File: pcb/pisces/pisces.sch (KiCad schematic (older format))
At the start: 41 parts, among them SW1 SW_PUSH, SW10 SW_PUSH, SW11 SW_PUSH, SW12 SW_PUSH, SW13 SW_PUSH, SW14 SW_PUSH, SW15 SW_PUSH, SW16 SW_PUSH, SW17 SW_PUSH, SW18 SW_PUSH, SW19 SW_PUSH, SW2 SW_PUSH, SW3 SW_PUSH, SW4 SW_PUSH, SW5 SW_PUSH, SW6 SW_PUSH, SW7 SW_PUSH, SW8 SW_PUSH, SW9 SW_PUSH, U1 ProMicro

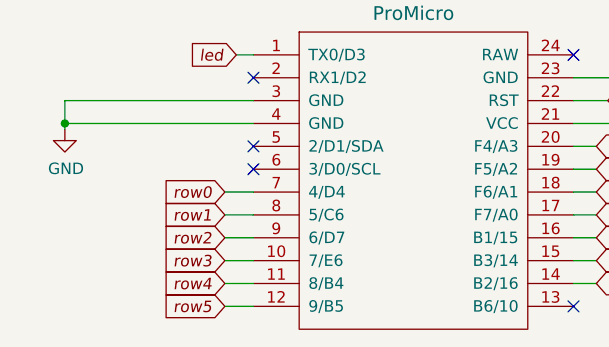
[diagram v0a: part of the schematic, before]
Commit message: Generated .net and .kicad_pcb
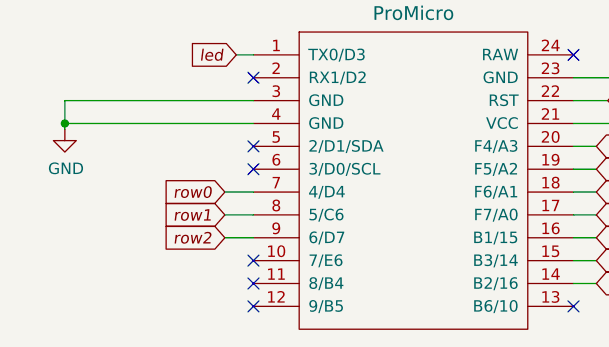
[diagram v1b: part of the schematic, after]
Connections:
- net row3: no longer names the net of U1.10 (7/E6)
- net row4: no longer names the net of U1.11 (8/B4)
- net row5: no longer names the net of U1.12 (9/B5)
- no-connect marks 6 -> 9
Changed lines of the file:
@@
 Pro Micro
-$Comp
-L kbd:ProMicro U1
-U 1 1 5FB09374
-P 2125 6925
-F 0 "U1" H 2125 7762 60  0000 C CNN
-F 1 "ProMicro" H 2125 7656 60  0000 C CNN
-F 2 "Keebio-Parts:ArduinoProMicro" H 2225 5875 60  0001 C CNN
-F 3 "" H 2225 5875 60  0000 C CNN
-	1    2125 6925
-	1    0    0    -1
-$EndComp
 $Comp
 L power:GND #PWR01
@@
 Text GLabel 1300 7175 0    50   Input Italic 0
 row2
-Text GLabel 1300 7275 0    50   Input Italic 0
-row3
-Text GLabel 1300 7375 0    50   Input Italic 0
-row4
-Text GLabel 1300 7475 0    50   Input Italic 0
-row5
 Text GLabel 2925 6775 2    50   Input Italic 0
 col0
@@
 Wire Wire Line
 	1300 7175 1425 7175
-Wire Wire Line
-	1300 7375 1425 7375
-Wire Wire Line
-	1300 7475 1425 7475
-Wire Wire Line
-	1300 7275 1425 7275
 NoConn ~ 2825 6375
 NoConn ~ 2825 7475
@@
 NoConn ~ 1425 6775
 NoConn ~ 1425 6475
+$Comp
+L kbd:ProMicro U1
+U 1 1 5FB09374
+P 2125 6925
+F 0 "U1" H 2125 7762 60  0000 C CNN
+F 1 "ProMicro" H 2125 7656 60  0000 C CNN
+F 2 "Keebio-Parts:ArduinoProMicro" H 2225 5875 60  0001 C CNN
+F 3 "" H 2225 5875 60  0000 C CNN
+	1    2125 6925
+	1    0    0    -1
+$EndComp
+NoConn ~ 1425 7275
+NoConn ~ 1425 7375
+NoConn ~ 1425 7475
 $EndSCHEMATC
